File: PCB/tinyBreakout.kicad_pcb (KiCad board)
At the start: 2 copper layers, 25.9 x 20.6 mm, 14 parts, among them IC1 ATTINY13A-S, P1 CONN_01X06, P2 CONN_01X02, P3 CONN_01X02, P4 CONN_01X02, U1 LD2979

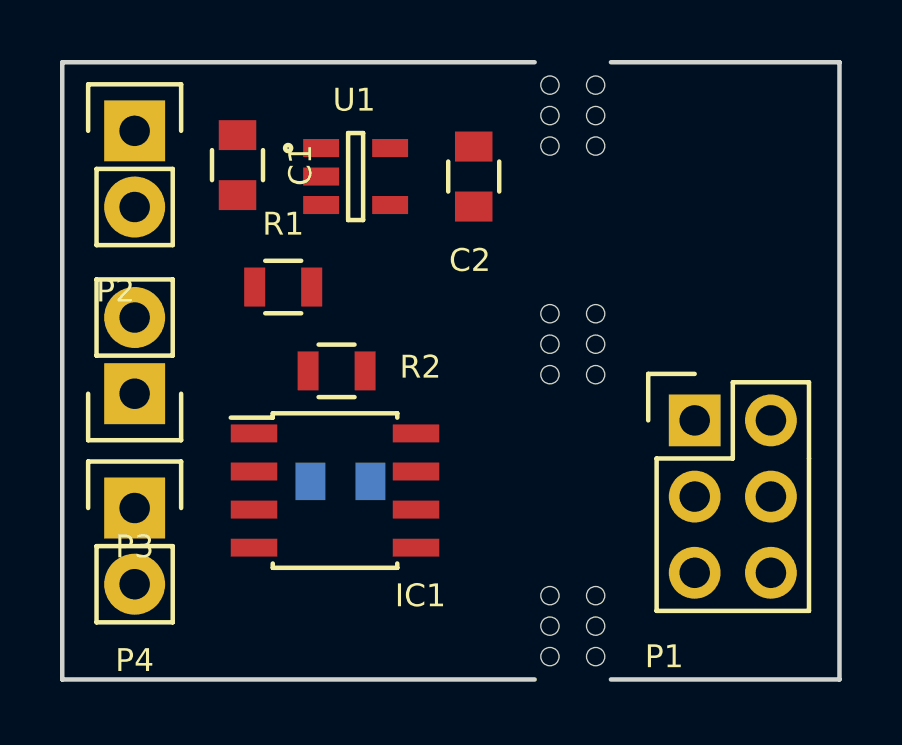
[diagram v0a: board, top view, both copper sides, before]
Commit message: Played around with the layout
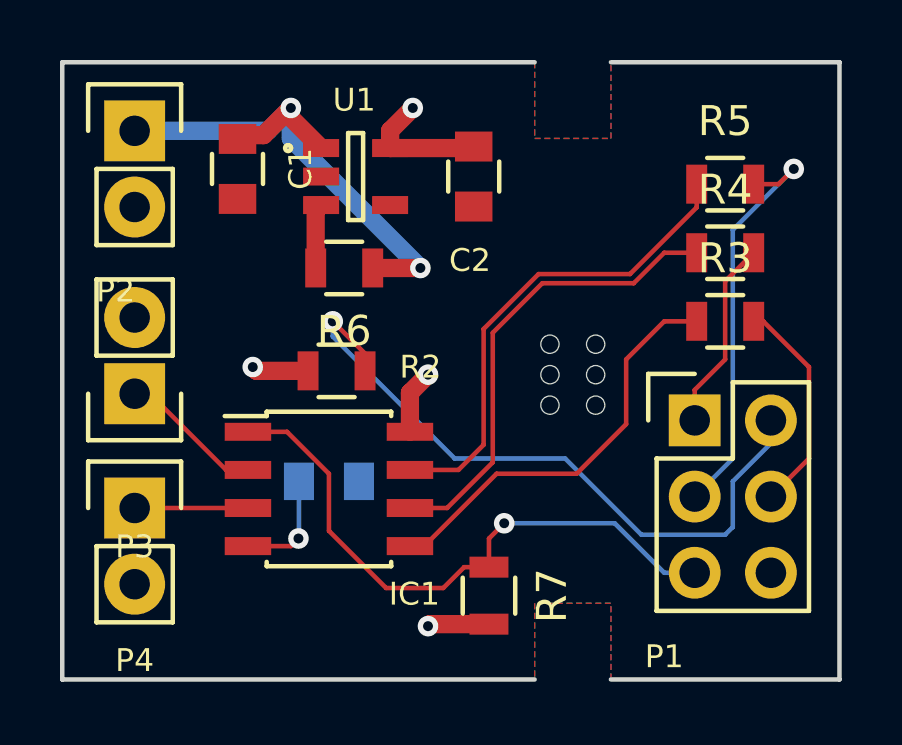
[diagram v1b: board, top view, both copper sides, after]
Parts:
- removed R1: 0Ω, Resistors_SMD:R_0805
- removed the REF** at (193.0, 103.9)
- removed the REF** at (193.0, 113.3)
- removed the REF** at (193.0, 96.3)
- added R3: 1kΩ, Resistors_SMD:R_0805, F.Cu at (198.9, 104.1)
- added R4: 1kΩ, Resistors_SMD:R_0805, F.Cu at (198.9, 101.9)
- added R5: 1kΩ, Resistors_SMD:R_0805, F.Cu at (198.9, 99.6)
- added R6: 0Ω, Resistors_SMD:R_0805, F.Cu at (186.2, 102.4)
- added R7: 10KΩ, Resistors_SMD:R_0805, F.Cu at (191.0, 113.3)
- added REF**: MouseBite, tinyBreakout:MouseBite, F.Cu at (193.0, 104.9)
- R2: value 10KΩ -> 1kΩ
- moved C3 0.38 mm to (185.7, 109.5)
- moved IC1 0.21 mm to (185.7, 109.7)
- moved C1 0.13 mm to (182.6, 99.1)
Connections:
- net /V+ renamed /Vin
- P1 pad 1: MISO -> Net-(P1-Pad1)
- P1 pad 2: Vcc -> Net-(P1-Pad2)
- P1 pad 3: SCK -> Net-(P1-Pad3)
- P1 pad 4: MOSI -> Net-(P1-Pad4)
- R2 pad 1: RESET -> Vcc
- R2 pad 2: Vcc -> Net-(P1-Pad2)
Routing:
- net Net-(P1-Pad2): track 0.00 -> 22.9 mm, vias 0 -> 1
- net RESET: track 0.00 -> 20.8 mm, vias 0 -> 1
- net /Vin: track 0.00 -> 18.1 mm, vias 0 -> 2
- net SCK: track 0.00 -> 16.2 mm
- net MISO: track 0.00 -> 15.6 mm
- net Net-(P1-Pad3): track 0.00 -> 14.1 mm, vias 0 -> 1
- net MOSI: track 0.00 -> 13.9 mm
- net Vcc: track 0.00 -> 10.6 mm, vias 0 -> 4
- net Net-(P1-Pad4): track 0.00 -> 7.32 mm
- net Net-(P1-Pad1): track 0.00 -> 6.40 mm
- net PB3: track 0.00 -> 4.83 mm
- net PB4: track 0.00 -> 3.78 mm
- net Net-(C3-Pad2): track 0.00 -> 3.70 mm, vias 0 -> 1
- net Net-(R6-Pad2): track 0.00 -> 2.17 mm
- added copper zone on F.Cu, net GND
- added copper zone on B.Cu, net Vcc
